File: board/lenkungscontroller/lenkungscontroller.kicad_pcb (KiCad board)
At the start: 2 copper layers, 53.2 x 68 mm, 34 parts, among them J1 Conn_01x03, J2 Conn_01x02_Female, J3 Conn_01x03, M1 Conn_01x02_Male, U1 TPS54360DDA, U2 SPX3819M5-L-3-3, U3 A4950E

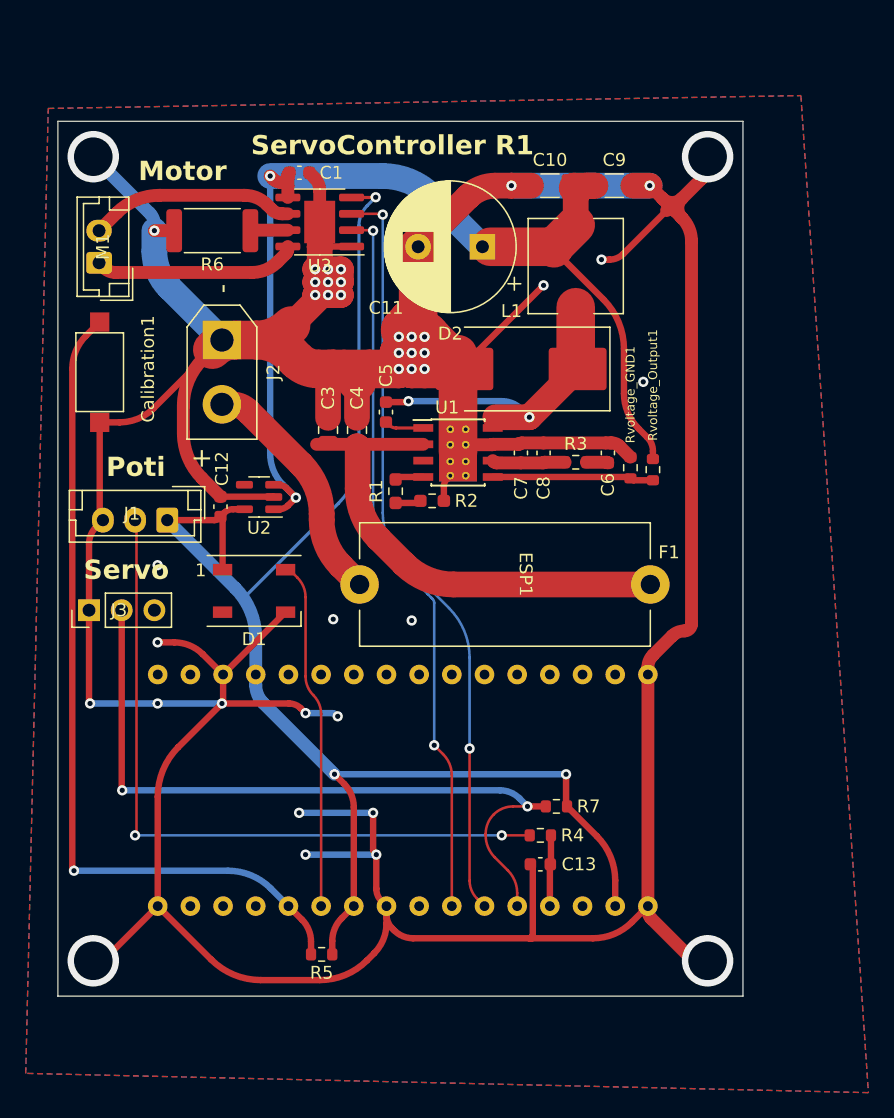
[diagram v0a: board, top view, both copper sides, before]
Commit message: updated steering controller
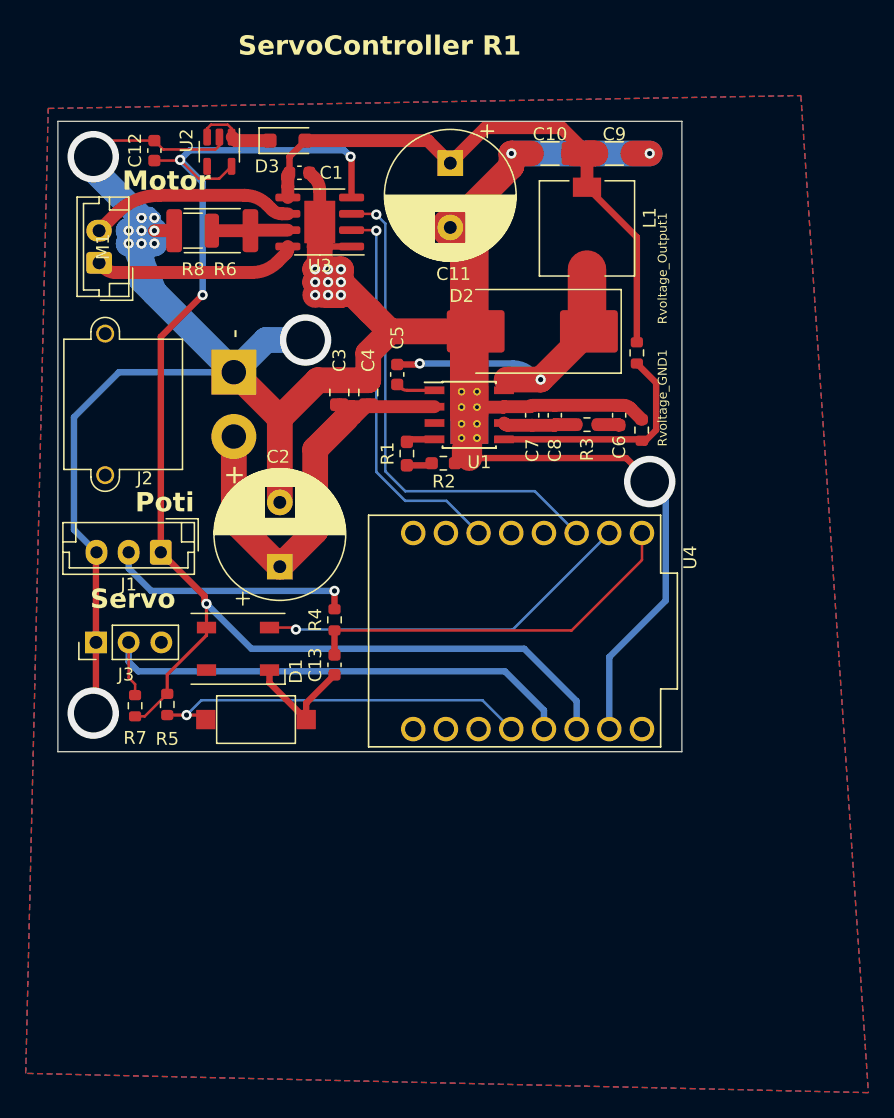
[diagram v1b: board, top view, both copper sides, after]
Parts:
- removed Calibration1: Boot, Button_Switch_SMD:SW_SPST_CK_RS282G05A3
- removed ESP1: ESP32, luatos-footprint:Luatos
- removed F1: Fuse, Fuse:Fuseholder_Cylinder-5x20mm_Stelvio-Kontek_PTF78_Horizontal_Open
- added Boot1: Boot, Button_Switch_SMD:SW_SPST_CK_RS282G05A3, F.Cu at (132.9, 87.5)
- added C2: 220uF, Capacitor_THT:CP_Radial_D10.0mm_P5.00mm, F.Cu at (134.8, 75.6)
- added D3: D, Diode_SMD:D_SOD-123F, F.Cu at (135.3, 42.5)
- added R8: 1.5, Resistor_SMD:R_1210_3225Metric, F.Cu at (128.0, 49.5)
- added U4: ESP32-C3_SUPERMINI, esp32c3supermini:MODULE_ESP32-C3_SUPERMINI, F.Cu at (153.0, 80.6)
- J2: footprint Connector_AMASS:AMASS_XT30UPB-M_1x02_P5.0mm_Vertical -> Connector_AMASS:AMASS_XT30PW-M_1x02_P2.50mm_Horizontal
- R6: value 0.25 -> 1.5
- moved R7 33.7 mm to (123.5, 86.4), turned to 90 degrees
- moved C12 28.1 mm to (125.0, 43.3)
- moved U2 27.0 mm to (130.1, 43.4), turned to -90 degrees
- moved R4 23.2 mm to (139.0, 79.8), turned to 90 degrees
- moved R5 22.8 mm to (126.0, 86.3), turned to -90 degrees
- moved C13 22.3 mm to (139.0, 83.2), turned to -90 degrees
- moved Rvoltage_Output1 9.16 mm to (162.5, 59.0)
- moved C11 6.96 mm to (148.0, 44.2), turned to -90 degrees
- moved D1 4.67 mm to (131.5, 82.0)
- moved C5 3.05 mm to (143.9, 60.7)
- moved C6 3.05 mm to (161.1, 63.9)
- moved C7 3.05 mm to (154.4, 63.9)
- moved C8 3.05 mm to (156.1, 63.9)
- moved C3 3.05 mm to (139.4, 62.1)
- moved C4 3.05 mm to (141.6, 62.1)
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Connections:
- net Net-(ESP1-IO10) renamed Signal_In
- J2 pad 2: Net-(J2-Pin_2) -> VIN
- R5 pad 2: Net-(ESP1-IO04) -> Calibrate
- U2 pad 1: 12V -> Net-(D3-K)
- U2 pad 3: 12V -> Net-(D3-K)
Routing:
- net GND: track 420.2 -> 264.8 mm, vias 41 -> 23
- net Net-(ESP1-IO04): track 65.3 -> 0.00 mm, vias 1 -> 0
- net 12V: track 86.7 -> 48.1 mm, vias 2 -> 0
- net Net-(J1-Pin_2): track 55.2 -> 19.4 mm, vias 2 -> 1
- net Calibrate: track 0.00 -> 29.8 mm, vias 0 -> 1
- net IN2: track 56.3 -> 30.6 mm, vias 2 -> 1
- net Poti: track 5.53 -> 30.2 mm
- net IN1: track 58.9 -> 39.0 mm, vias 2 -> 1
- net Net-(J2-Pin_2): track 18.7 -> 0.00 mm
- net Signal_In: track 58.2 -> 41.1 mm, vias 2 -> 0
- net 3_3V: track 117.1 -> 107.6 mm, vias 3 -> 4
- net Net-(D3-K): track 0.00 -> 6.49 mm
- net Net-(U1-FB): track 12.5 -> 18.3 mm
- net Net-(U3-LSS): track 2.93 -> 5.93 mm
- net VIN: track 38.2 -> 35.3 mm
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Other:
- board size 53.2 x 68 mm -> 48.5 x 49 mm
